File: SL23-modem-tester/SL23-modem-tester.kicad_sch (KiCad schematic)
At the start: 12 parts, among them J1 691322310002

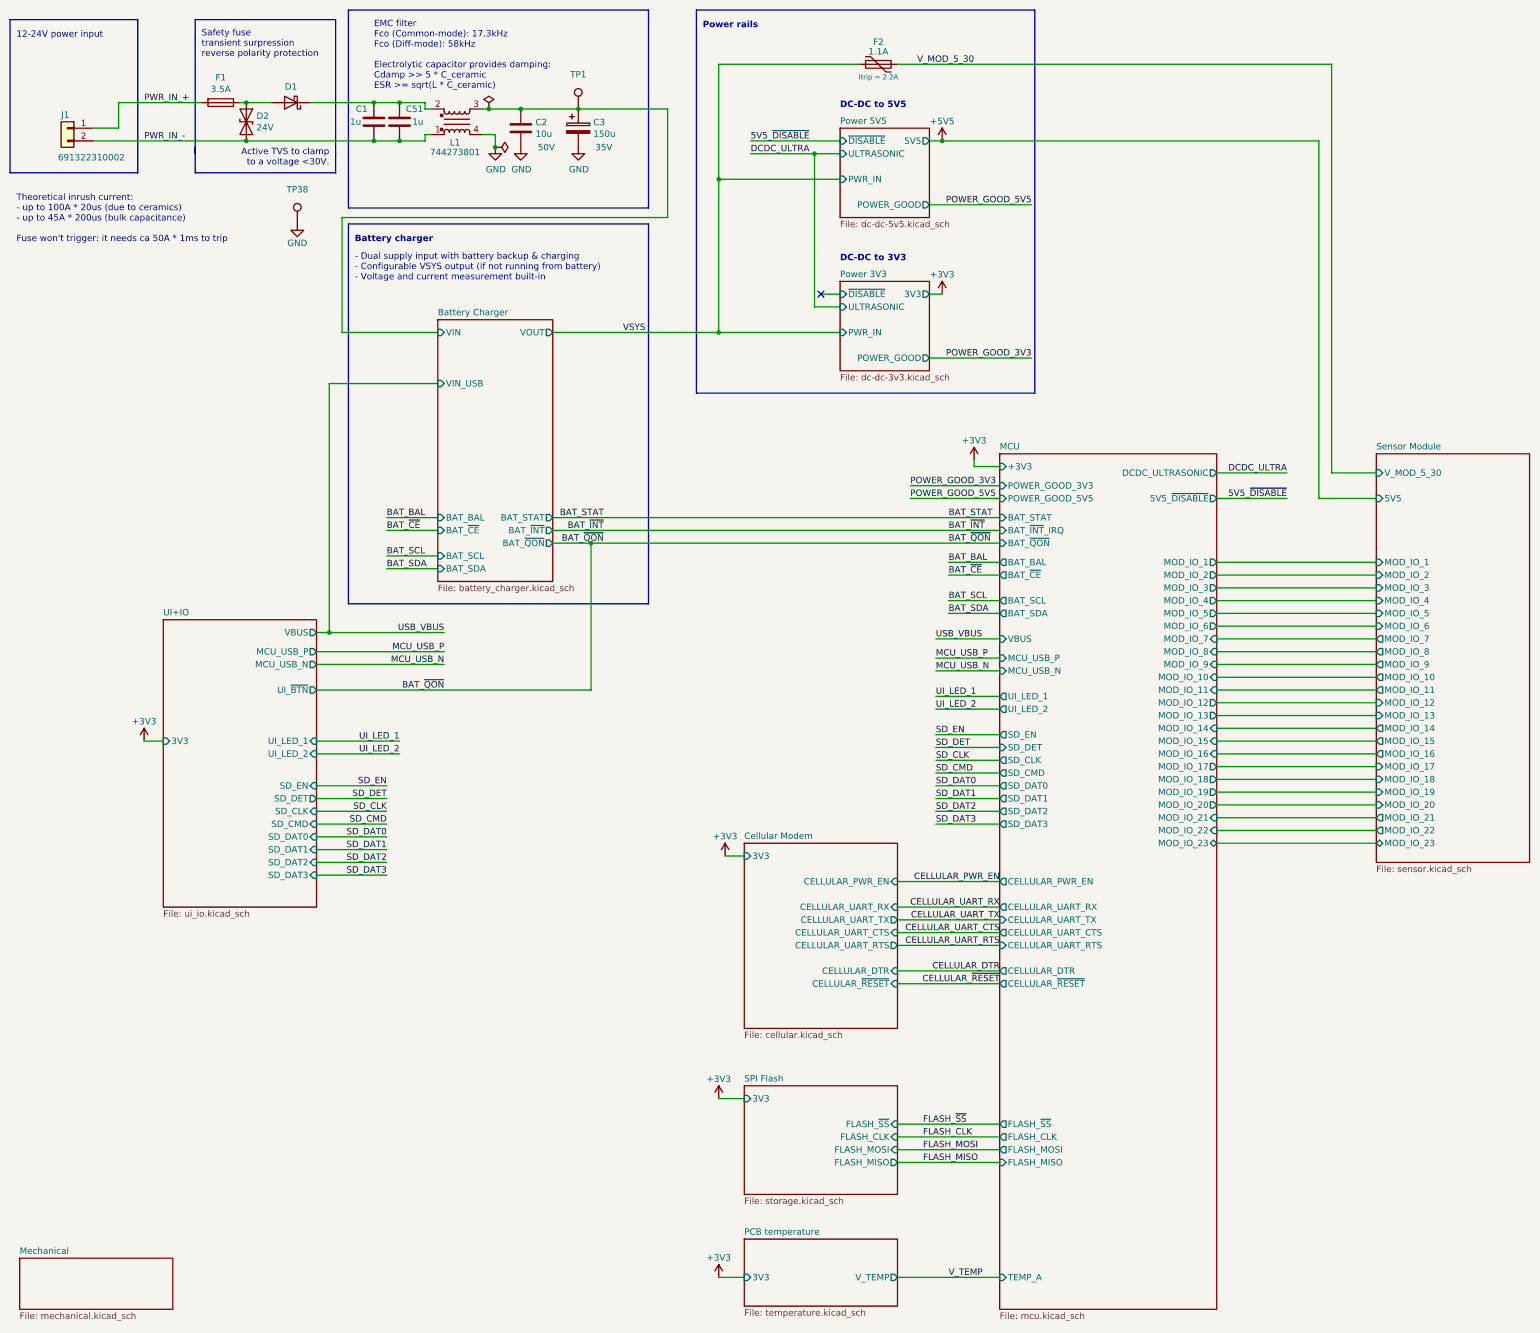
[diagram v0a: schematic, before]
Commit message: SL23-modem-tester: release after manual review
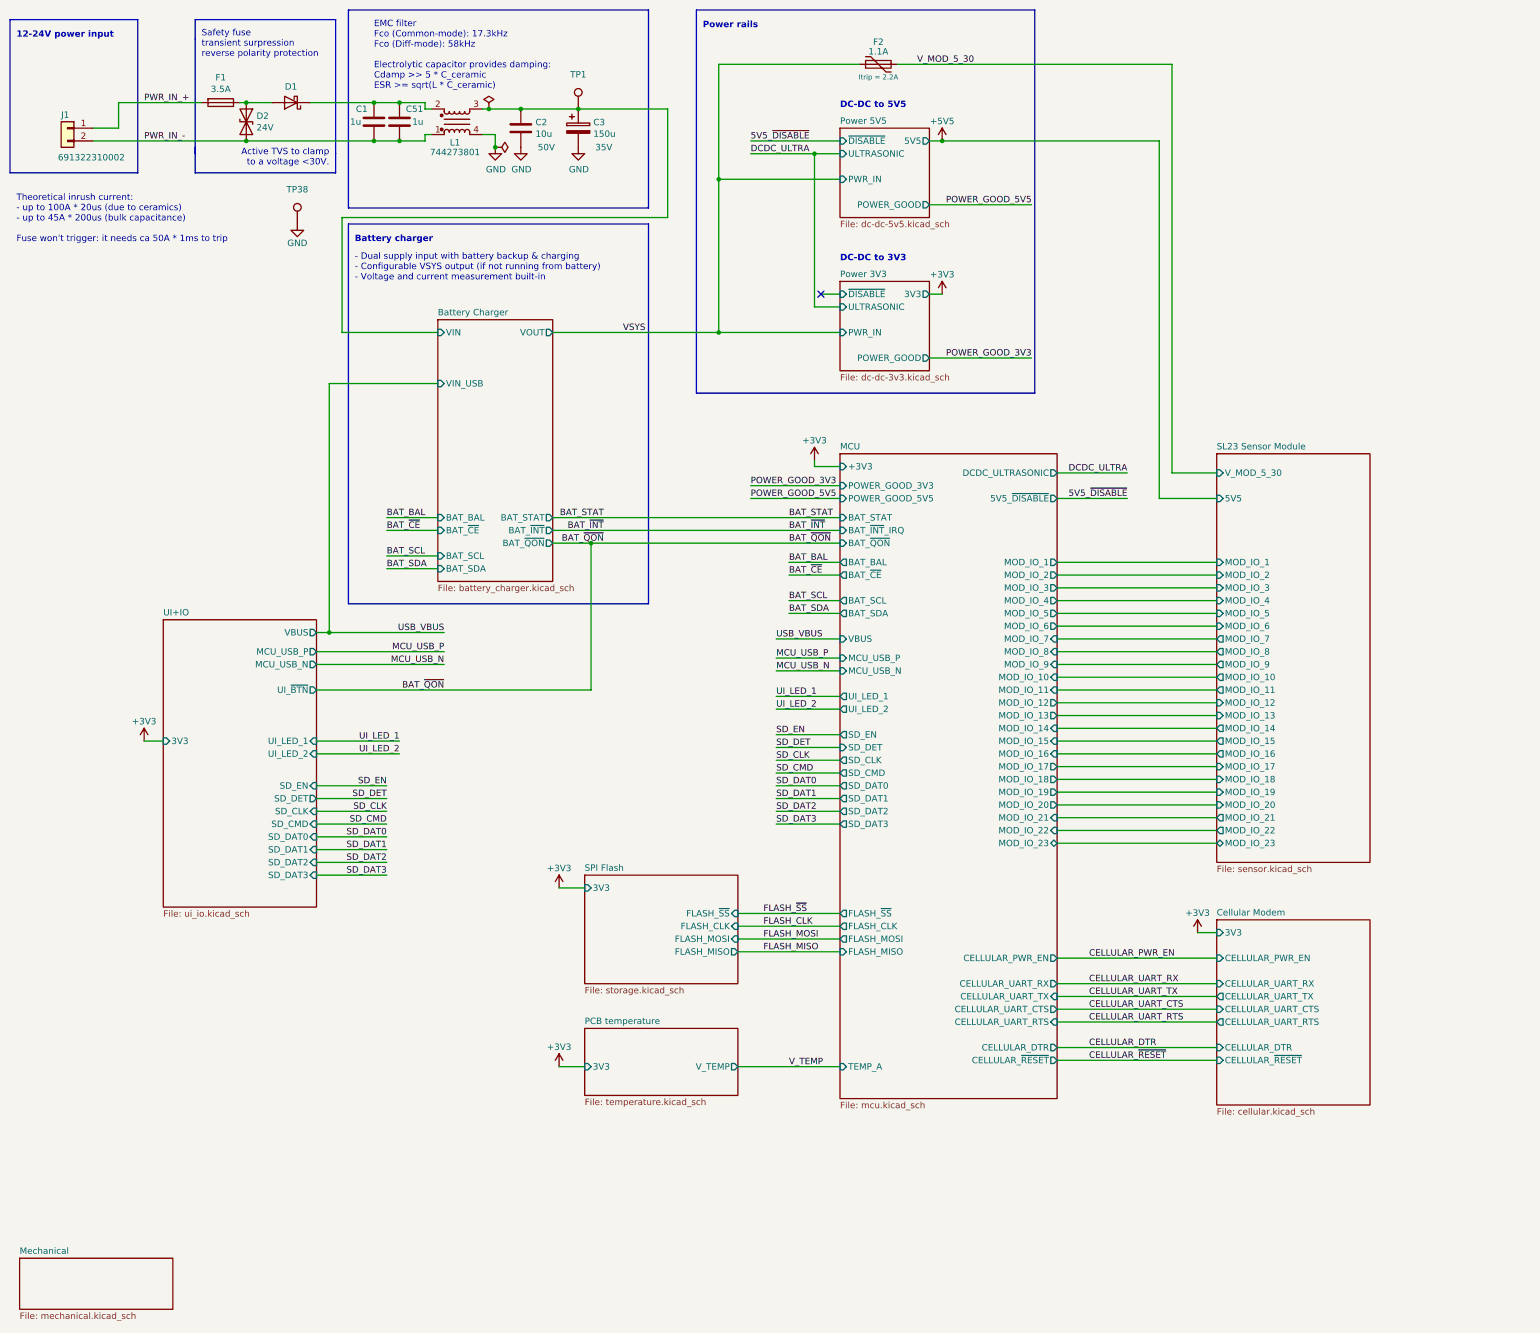
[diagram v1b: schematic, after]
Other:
- sheet Sensor Module renamed SL23 Sensor Module
